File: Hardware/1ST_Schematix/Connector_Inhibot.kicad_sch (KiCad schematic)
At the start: 13 parts, among them J501 Conn_01x06, J503 Conn_01x06, J504 Conn_01x05, J506 Conn_01x03, J507 Conn_01x03, J508 Conn_01x06, J509 Conn_01x06, J510 Conn_01x06, J511 Conn_01x03, U501 SN74AHCT1G125DBVR

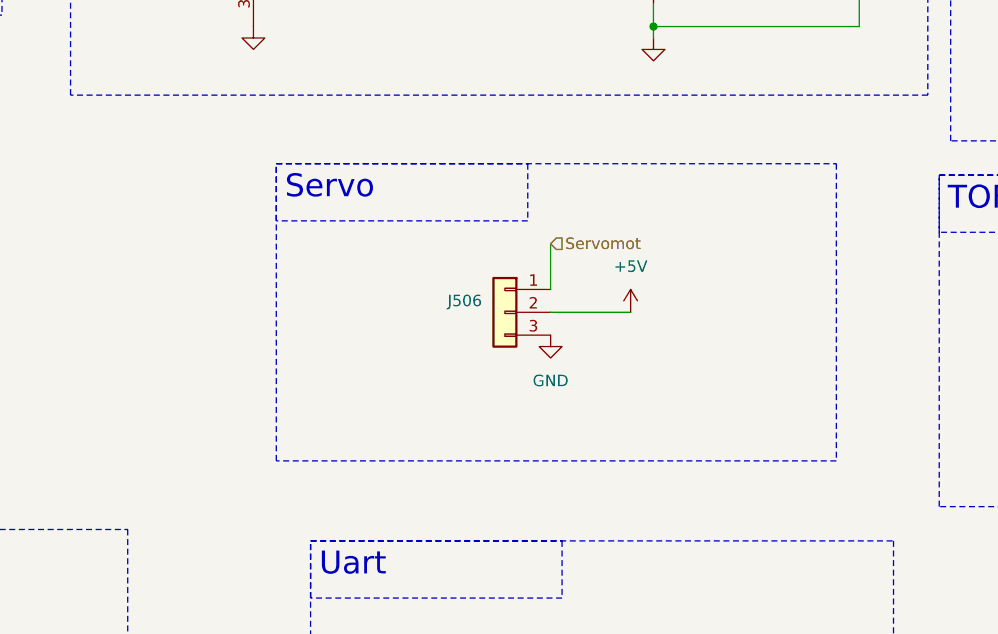
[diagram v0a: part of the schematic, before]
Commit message: routage à faire vérifier
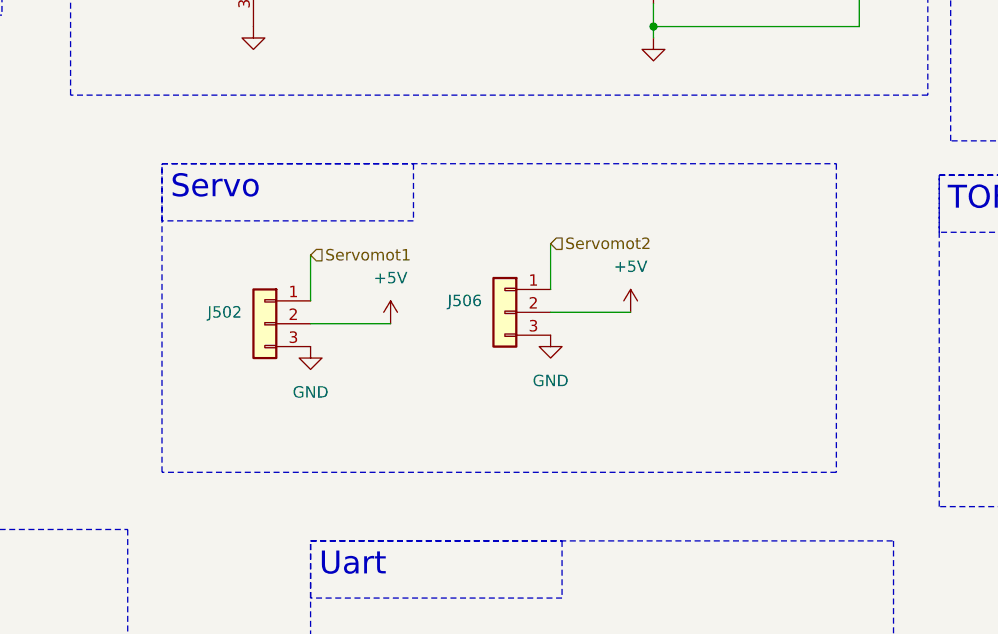
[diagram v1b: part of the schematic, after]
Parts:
- added J502: Conn_01x03, Connector_JST:JST_EH_B3B-EH-A_1x03_P2.50mm_Vertical, symbol Connector_Generic:Conn_01x03
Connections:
- net +5V: now also J502.2 (Pin_2)
- net GND: now also J502.3 (Pin_3)
- net Servomot renamed Servomot2
- new net Servomot1: J502.1 (Pin_1)
